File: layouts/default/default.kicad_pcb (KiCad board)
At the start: 2 copper layers, 88 x 62 mm, 62 parts, among them U10 10µF ±10% 25V X5R, U11 10µF ±10% 25V X5R, U12 10µF ±10% 25V X5R, U13 1MΩ ±1% 62.5mW, U14 100nF ±10% 16V X7R, U16 1µF ±10% 25V X5R, U17 560Ω ±1% 62.5mW, U18 1µF ±10% 25V X5R, U19 4.7kΩ ±1% 62.5mW, U20 10µF ±10% 25V X5R, U21 10µF ±10% 25V X5R, U23 10kΩ ±1% 62.5mW, U25 100nF ±10% 16V X7R, U29 4.7kΩ ±1% 62.5mW, U5 820Ω ±1% 62.5mW, U6 4.7kΩ ±1% 62.5mW, U8 1.5µH ±20%, U9 10µF ±10% 25V X5R

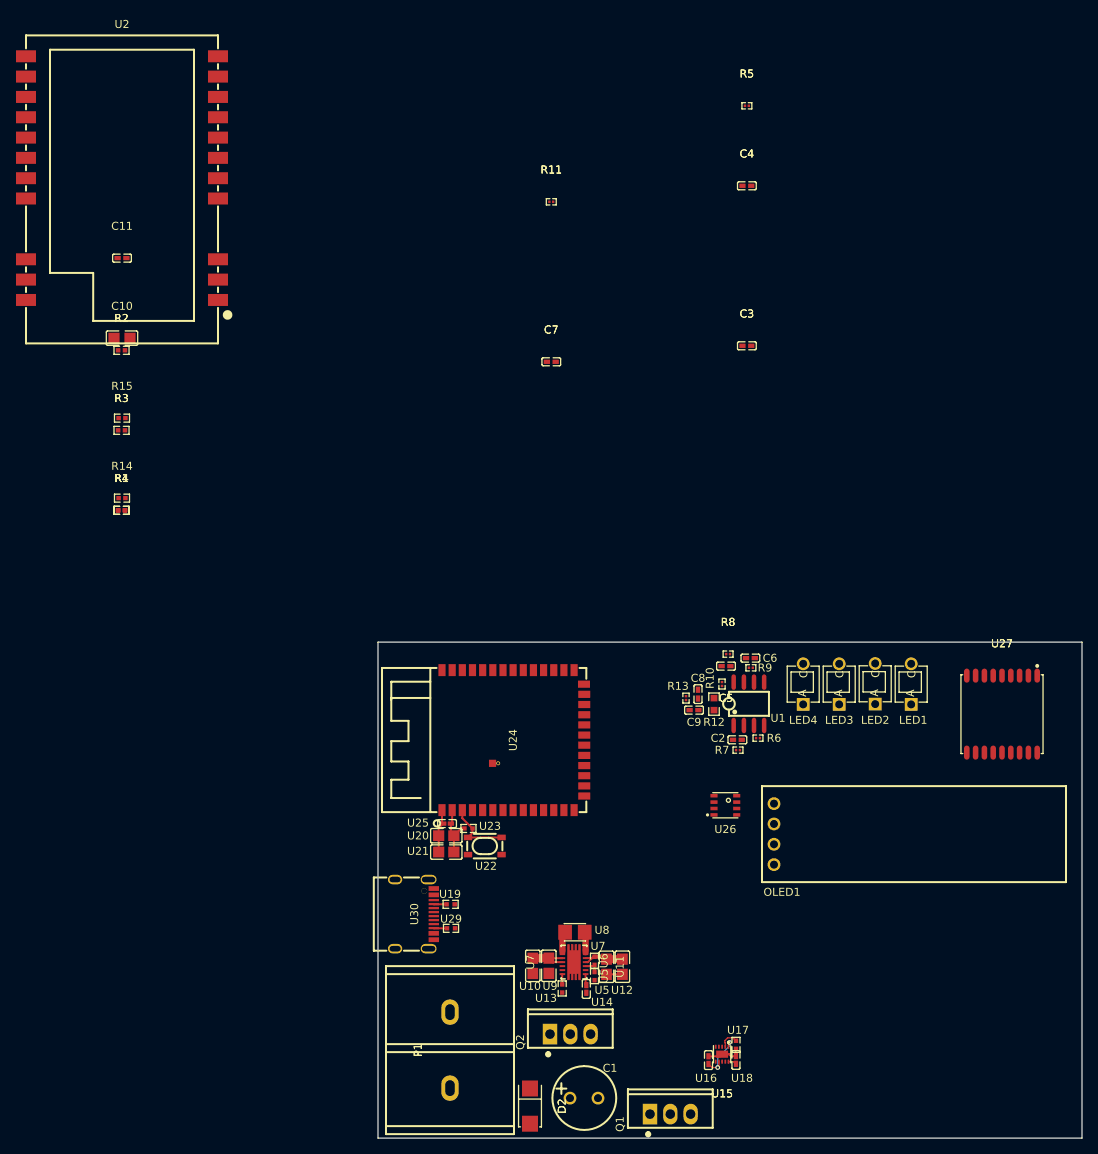
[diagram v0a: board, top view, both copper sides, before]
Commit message: layout updates
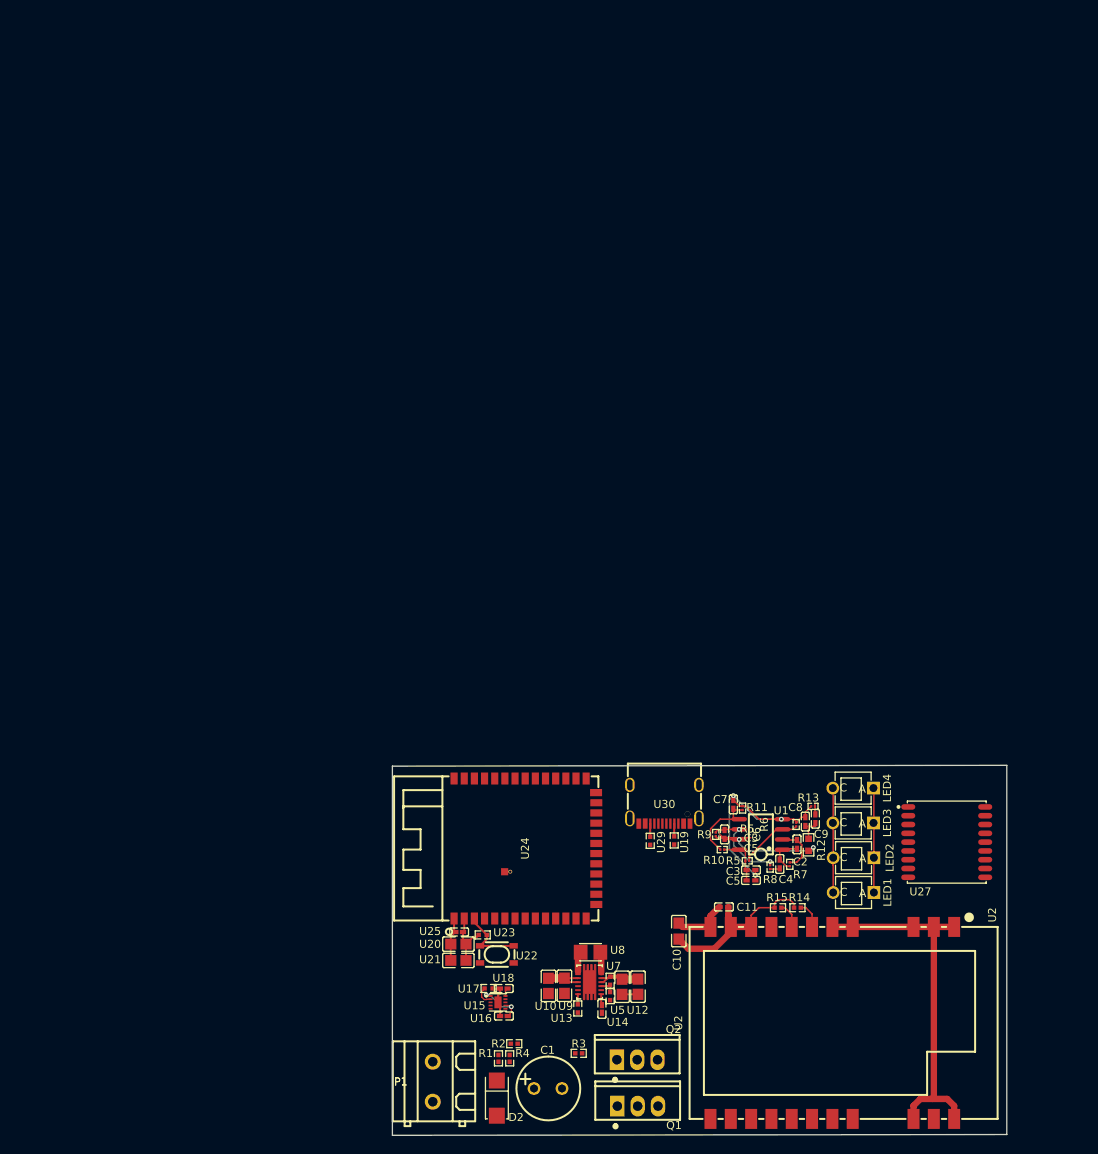
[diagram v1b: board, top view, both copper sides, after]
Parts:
- removed OLED1: , atopile:OLED-TH_L38.0-W12.0_HS91L02W2C01-1fd193
- removed U26: , atopile:LGA-8_L3.0-W3.0-P0.80_BME688-7465bb
- P1: footprint atopile:CONN-TH_2P-P9.50_WJ45C-B-2P-7aea0b -> atopile:CONN-TH_2P-P5.00_WJ128V-5.0-2P-75f14f
- moved U2 138.0 mm to (88.8, 65.6), turned to 90 degrees
- moved C11 110.6 mm to (75.2, 51.1), turned to 180 degrees
- moved R15 102.3 mm to (82.0, 51.2)
- moved C10 101.7 mm to (69.6, 54.1), turned to 90 degrees
- moved R2 99.6 mm to (49.0, 68.2)
- moved R14 98.7 mm to (84.4, 51.2)
- moved R3 96.6 mm to (57.1, 69.4), turned to 180 degrees
- moved R5 94.4 mm to (78.2, 45.3)
- moved C4 84.9 mm to (82.2, 45.7), turned to -90 degrees
- moved R4 83.9 mm to (48.5, 70.0), turned to 90 degrees
- moved R1 83.1 mm to (47.1, 70.0), turned to -90 degrees
- moved R11 79.5 mm to (77.6, 38.7), turned to 90 degrees
- moved C3 65.5 mm to (78.6, 46.5)
- moved C7 59.8 mm to (76.4, 38.3), turned to 90 degrees
- moved U30 34.1 mm to (67.8, 38.3), turned to 180 degrees
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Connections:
- net B5 renamed CC2
- net CC1 renamed A5
- net DN1 renamed DN2
- net DP1 renamed DP2
- C10 pad 1: hv -> hv-2
- C11 pad 1: hv -> hv-2
- C3 pad 1: hv -> hv-2
- C4 pad 2: detector-net-1 -> detector-net
- C5 pad 1: hv -> hv-2
- C8 pad 1: detector-net -> detector-net-1
- C9 pad 1: detector-net -> detector-net-1
- R1 pad 1: hv -> hv-2
- R10 pad 1: hv -> hv-2
- R12 pad 2: detector-net -> detector-net-1
- R14 pad 1: hv -> hv-2
- R15 pad 1: hv -> hv-2
- R5 pad 1: hv -> hv-2
- R8 pad 1: detector-net-1 -> detector-net
- U1 pad 8: hv -> hv-2
- U10 pad 1: hv-3 -> hv
- U11 pad 1: hv -> hv-2
- U12 pad 1: hv -> hv-2
- U15 pad 1: hv-2 -> hv-1
- U15 pad 10: hv-3 -> hv
- U15 pad 7: hv-2 -> hv-1
- U16 pad 1: hv-2 -> hv-1
- U18 pad 1: hv-3 -> hv
- U2 pad 10: hv -> hv-2
- U2 pad 9: hv -> hv-2
- U20 pad 1: hv-1 -> hv-3
- U21 pad 1: hv-1 -> hv-3
- U23 pad 1: hv-1 -> hv-3
- U24 pad 2: hv-1 -> hv-3
- U24 pad 3: EN -> in
- U25 pad 1: hv-1 -> hv-3
- U27 pad 14: hv-1 -> hv-3
- U27 pad 8: hv-1 -> hv-3
- U30 pad A4: hv-2 -> hv-1
- U30 pad A9: hv-2 -> hv-1
- U30 pad B4: hv-2 -> hv-1
- U30 pad B9: hv-2 -> hv-1
- U6 pad 1: hv -> hv-2
- U7 pad 10: hv-3 -> hv
- U7 pad 11: hv-3 -> hv
- U7 pad 4: hv -> hv-2
- U7 pad 5: hv -> hv-2
- U9 pad 1: hv-3 -> hv
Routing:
- net gnd: track 12.0 -> 110.4 mm, vias 0 -> 3
- net hv-2: track 6.47 -> 36.4 mm, vias 2 -> 0
- net detector-K: track 0.00 -> 19.1 mm
- net OUT2: track 0.00 -> 17.4 mm, vias 0 -> 2
- net IN2minus: track 0.00 -> 11.3 mm, vias 0 -> 2
- net IN2plus: track 0.00 -> 10.4 mm
- net IN1plus: track 0.00 -> 7.96 mm
- net hv: track 0.00 -> 6.80 mm
- net (no net): track 6.20 -> 0.00 mm
- net OUT1: track 0.00 -> 5.03 mm
- net RXEN: track 0.00 -> 4.05 mm
- net TXEN: track 0.00 -> 3.23 mm
- net detector-net-1: track 0.00 -> 2.82 mm
- net out: track 0.00 -> 1.42 mm
- net detector-net: track 0.00 -> 1.23 mm
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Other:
- board size 88 x 62 mm -> 76.8 x 46.3 mm
